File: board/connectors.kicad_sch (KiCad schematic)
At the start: 7 parts, among them J2 Power, J3 Connections, J4 LED

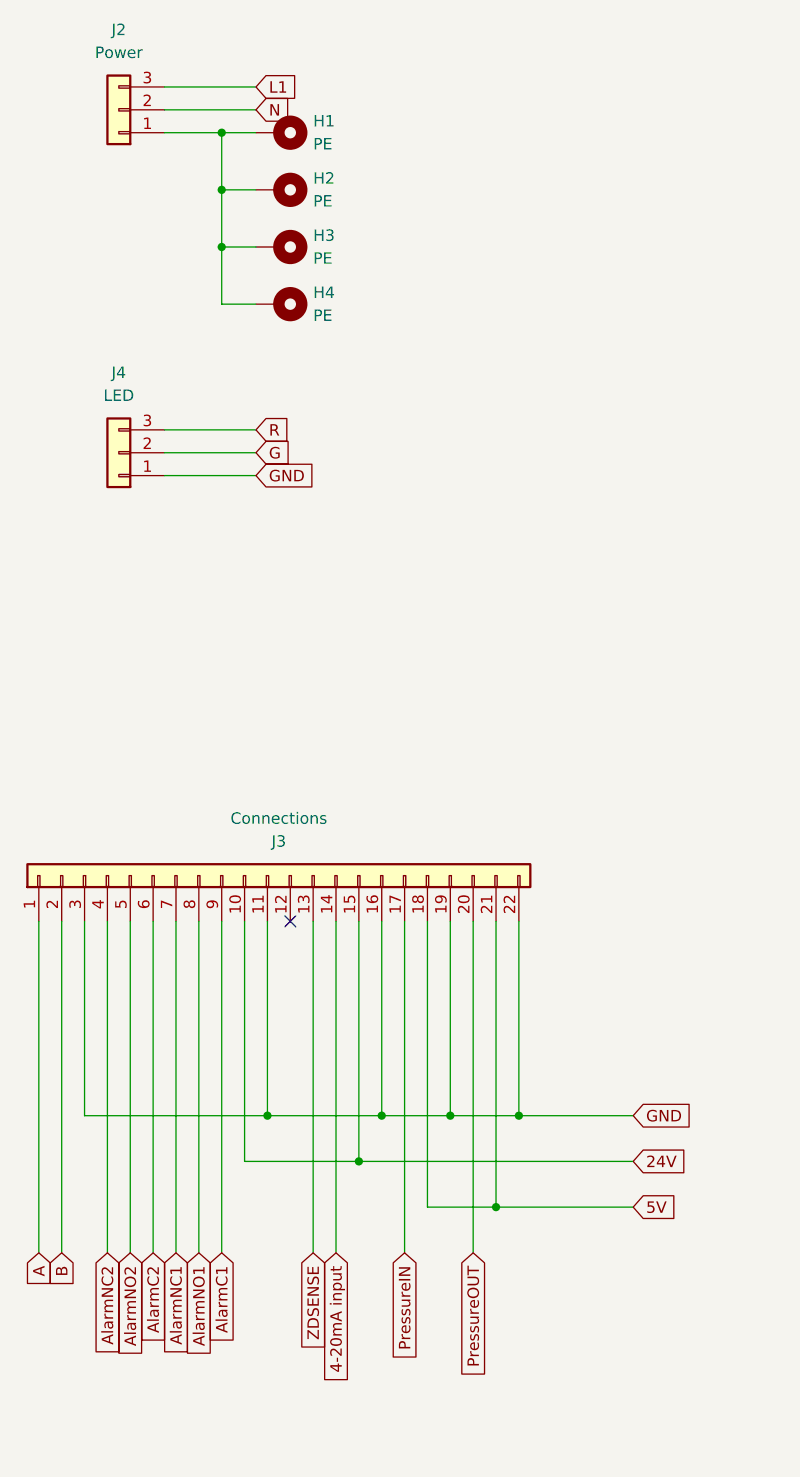
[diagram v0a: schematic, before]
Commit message: Power shit and copper fillz boi
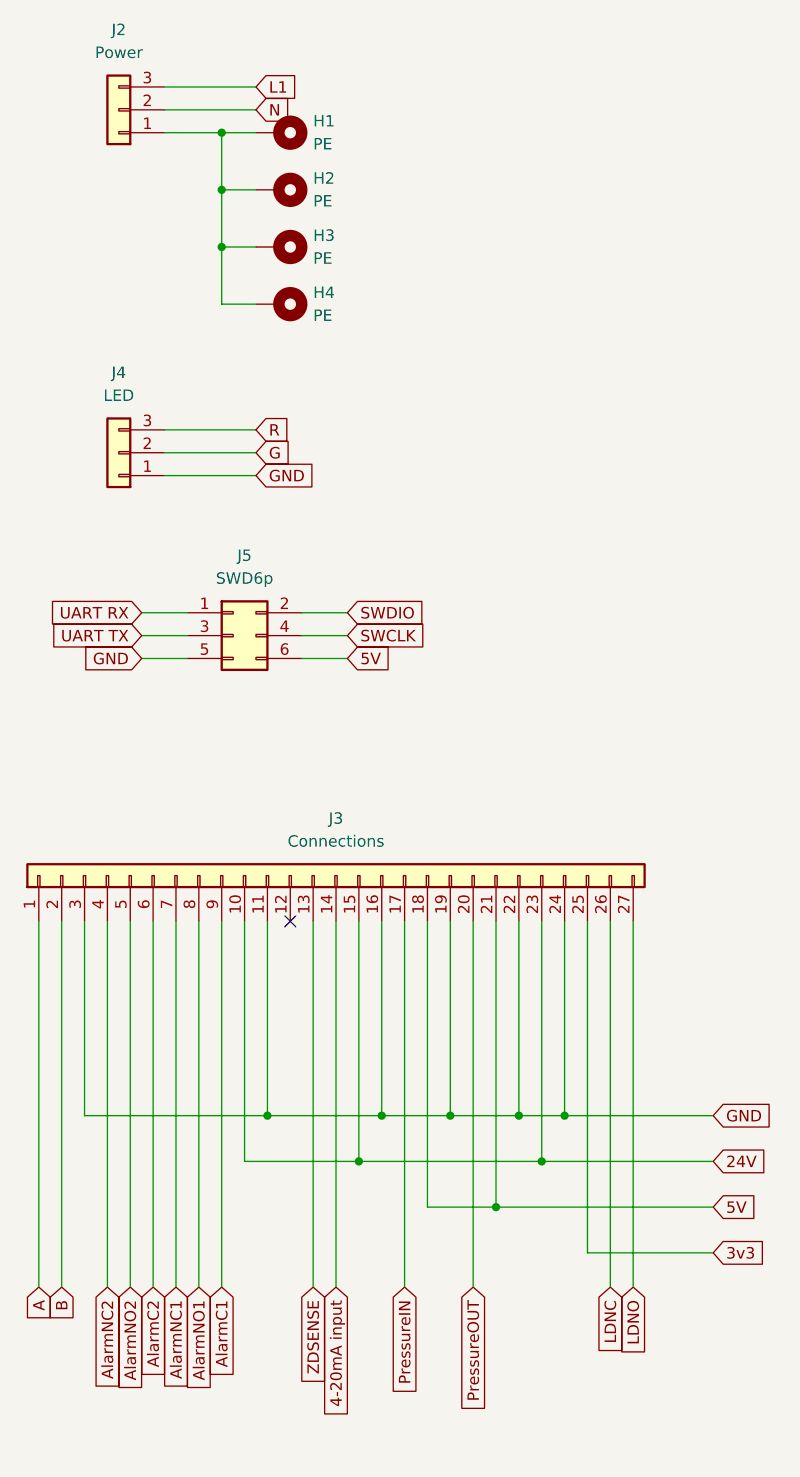
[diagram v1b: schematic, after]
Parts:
- removed J3: Connections, Connector_PinHeader_2.54mm:PinHeader_1x22_P2.54mm_Vertical, symbol Connector_Generic:Conn_01x22
- added J3: Connections, Connector_PinHeader_2.54mm:PinHeader_1x27_P2.54mm_Vertical, symbol Connector_Generic:Conn_01x27
- added J5: SWD6p, Connector_PinHeader_2.54mm:PinHeader_2x03_P2.54mm_Vertical, symbol Connector_Generic:Conn_02x03_Odd_Even
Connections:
- net 24V: now also J3.10 (Pin_10), J3.15 (Pin_15), J3.23 (Pin_23)
- net 4-20mA input: now also J3.14 (Pin_14)
- net 5V: now also J3.18 (Pin_18), J3.21 (Pin_21), J5.6 (Pin_6)
- net A: now also J3.1 (Pin_1)
- net AlarmC1: now also J3.9 (Pin_9)
- net AlarmC2: now also J3.6 (Pin_6)
- net AlarmNC1: now also J3.7 (Pin_7)
- net AlarmNC2: now also J3.4 (Pin_4)
- net AlarmNO1: now also J3.8 (Pin_8)
- net AlarmNO2: now also J3.5 (Pin_5)
- net B: now also J3.2 (Pin_2)
- net GND: now also J3.11 (Pin_11), J3.16 (Pin_16), J3.19 (Pin_19), J3.22 (Pin_22), J3.24 (Pin_24), J3.3 (Pin_3), J5.5 (Pin_5)
- net PressureIN: now also J3.17 (Pin_17)
- net PressureOUT: now also J3.20 (Pin_20)
- net ZDSENSE: now also J3.13 (Pin_13)
- new net 3v3: J3.25 (Pin_25)
- new net LDNC: J3.26 (Pin_26)
- new net LDNO: J3.27 (Pin_27)
- new net SWCLK: J5.4 (Pin_4)
- new net SWDIO: J5.2 (Pin_2)
- new net UART RX: J5.1 (Pin_1)
- new net UART TX: J5.3 (Pin_3)
